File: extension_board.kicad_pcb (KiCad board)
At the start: 2 copper layers, 85.7 x 123.2 mm, 37 parts, among them CN1 Conn_02x20_Odd_Even, J1 Screw_Terminal_01x02, J2 Conn_01x02, J3 Conn_01x02, J4 Conn_01x02, J5 Conn_02x03_Odd_Even, J6 Conn_01x02, J7 Conn_02x14_Odd_Even, J8 Conn_02x10_Odd_Even, J9 Conn_02x19_Odd_Even, U1 LM334Z, U2 LM334Z, U3 LM334Z, U4 LM334Z

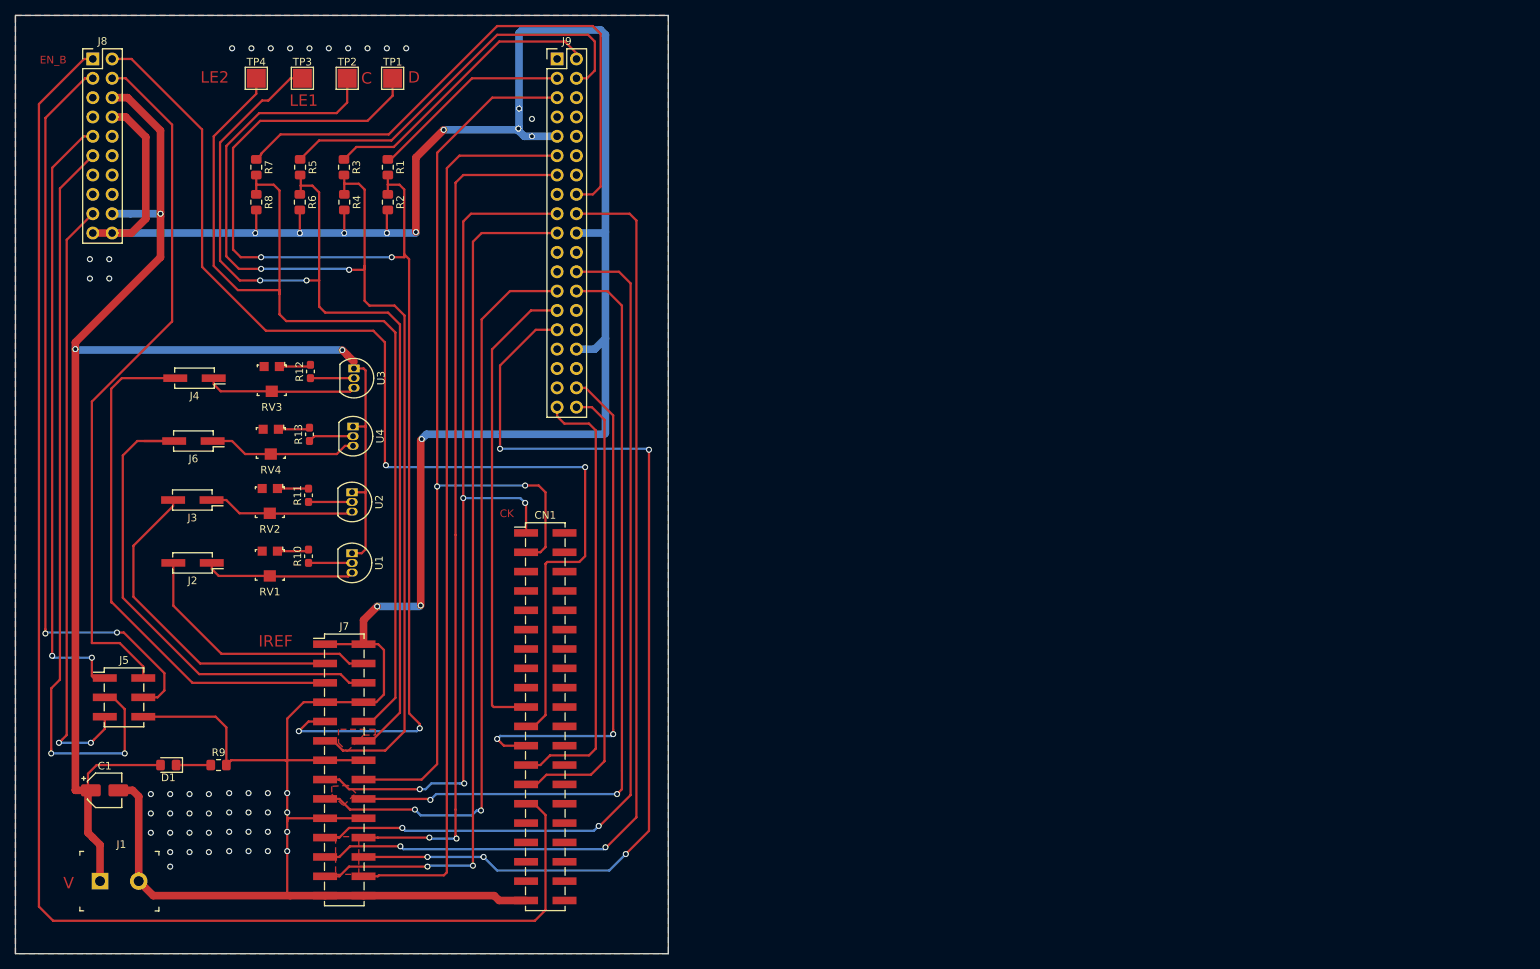
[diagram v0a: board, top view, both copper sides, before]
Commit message: gerber files and final files
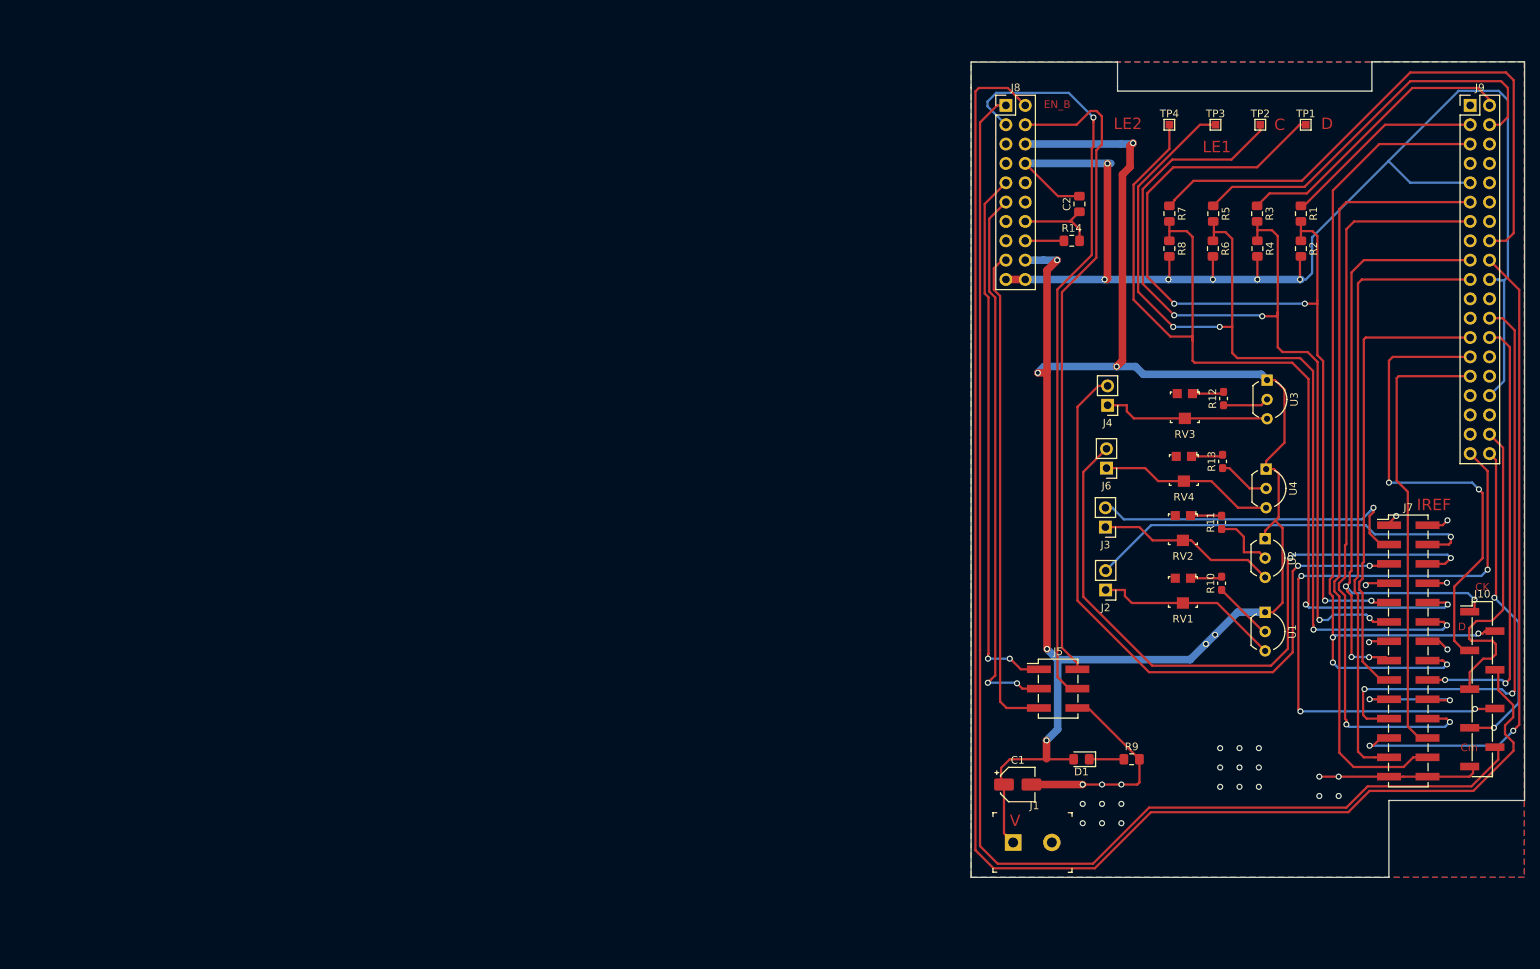
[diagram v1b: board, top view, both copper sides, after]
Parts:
- removed CN1: Conn_02x20_Odd_Even, Connector_PinHeader_2.54mm:PinHeader_2x20_P2.54mm_Vertical_SMD
- added C2: 1u, Capacitor_SMD:C_0805_2012Metric_Pad1.15x1.40mm_HandSolder, F.Cu at (91.4, 59.7)
- added J10: Conn_01x09_Male, Connector_PinHeader_2.54mm:PinHeader_1x09_P2.54mm_Vertical_SMD_Pin1Left, F.Cu at (144.3, 123.4)
- added R14: 10K, Resistor_SMD:R_0805_2012Metric_Pad1.15x1.40mm_HandSolder, F.Cu at (90.4, 64.5)
- J2, J3, J4, J6: footprint Connector_PinHeader_2.54mm:PinHeader_2x01_P2.54mm_Vertical_SMD -> Connector_PinHeader_2.54mm:PinHeader_1x02_P2.54mm_Vertical
- TP1, TP2, TP3, TP4: footprint TestPoint:TestPoint_Pad_2.5x2.5mm -> TestPoint:TestPoint_Pad_1.0x1.0mm
- U1, U2, U3, U4: footprint Package_TO_SOT_THT:TO-92_Inline -> Package_TO_SOT_THT:TO-92_Inline_Wide
- moved J7 140.6 mm to (134.6, 118.4)
- moved J5 122.7 mm to (88.6, 123.3)
- moved U1 120.1 mm to (115.8, 113.3)
- moved J8 120.0 mm to (81.8, 46.7)
- moved R4 120.0 mm to (114.8, 65.5)
- moved R7 120.0 mm to (103.3, 61.0)
- moved R8 120.0 mm to (103.3, 65.5)
- moved TP1 120.0 mm to (121.2, 49.3)
- moved TP3 120.0 mm to (109.3, 49.3)
- moved TP4 120.0 mm to (103.3, 49.3)
- moved U2 120.0 mm to (115.8, 103.6)
- moved J9 120.0 mm to (142.7, 46.7)
- moved R1 120.0 mm to (120.5, 61.0)
- moved R2 120.0 mm to (120.5, 65.5)
- moved R3 120.0 mm to (114.8, 61.0)
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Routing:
- net GND: track 412.2 -> 261.0 mm, vias 43 -> 27
- net SPI_MOSI: track 130.4 -> 59.3 mm, vias 5 -> 0
- net EN_SUP2: track 144.6 -> 197.6 mm, vias 2 -> 0
- net SW2_VCTRL: track 105.1 -> 58.0 mm
- net SPI_NSS: track 130.0 -> 86.4 mm
- net 3v3_POW_EN: track 117.9 -> 78.5 mm
- net IC_DATA_1v: track 160.3 -> 121.1 mm
- net VDD: track 201.2 -> 238.0 mm, vias 19 -> 17
- net SW1_VCTRL: track 97.6 -> 61.3 mm, vias 2 -> 0
- net SYNTH_POW_EN: track 113.4 -> 81.2 mm, vias 2 -> 0
- net PF7: track 99.5 -> 71.8 mm
- net I2C_CLK: track 118.1 -> 91.8 mm
- net IC_CLK_1v: track 148.0 -> 121.8 mm, vias 2 -> 4
- net EN_SUP4: track 58.9 -> 84.7 mm, vias 0 -> 4
- net EN_SUP3: track 67.9 -> 42.4 mm, vias 2 -> 0
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- added copper zone on B.Cu, net GND
- added copper zone on F.Cu, net VDD
- removed copper zone on F.Cu, net GND
- removed copper zone on B.Cu, net VDD
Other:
- board size 85.7 x 123.2 mm -> 72.7 x 107.1 mm
- board text added: "Cm"
